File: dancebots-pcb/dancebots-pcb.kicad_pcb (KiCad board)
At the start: 2 copper layers, 50 x 50 mm, 33 parts, among them J1 BATTERY, J2 MOT2-L, J3 MOT1-R, J4 MP3 Player, U1 L4941, U2 L293, U3 ATTINY261A-P, U4 LM386, U5 LM358

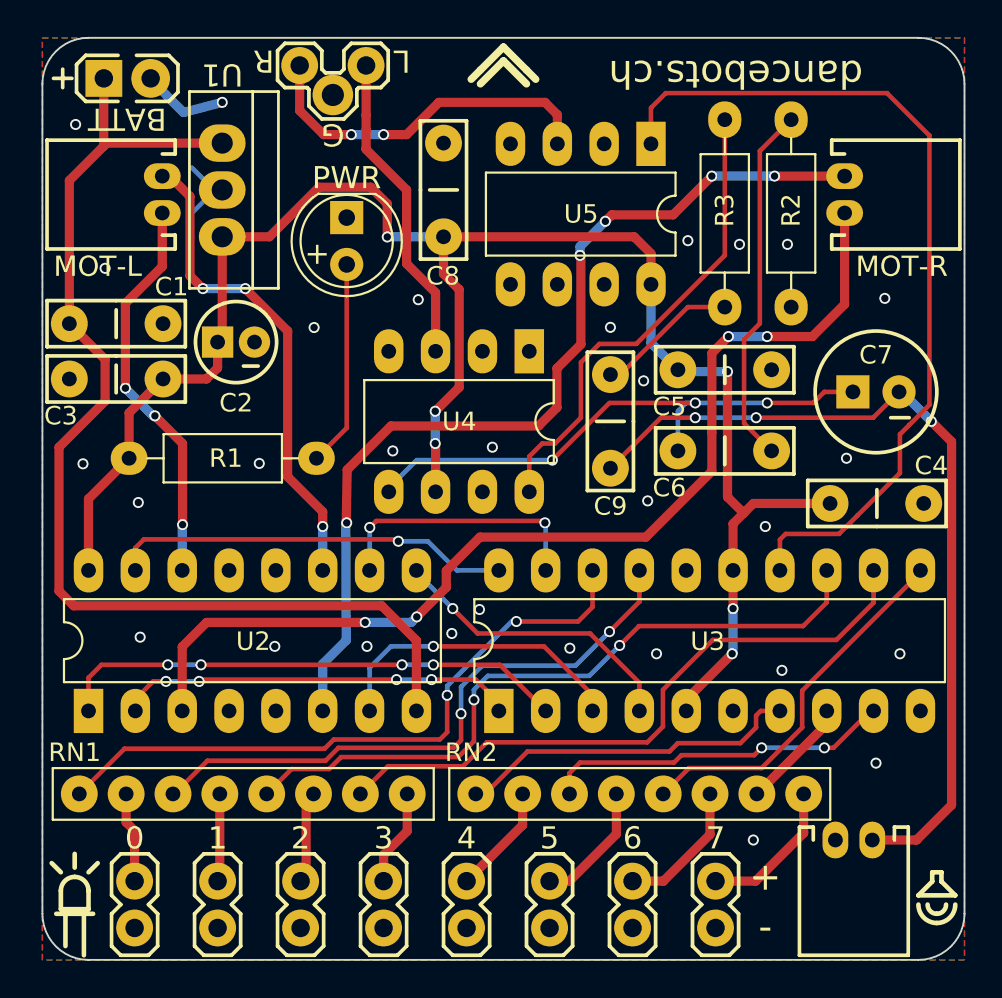
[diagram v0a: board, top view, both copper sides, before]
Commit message: migrated to Kicad 6.0
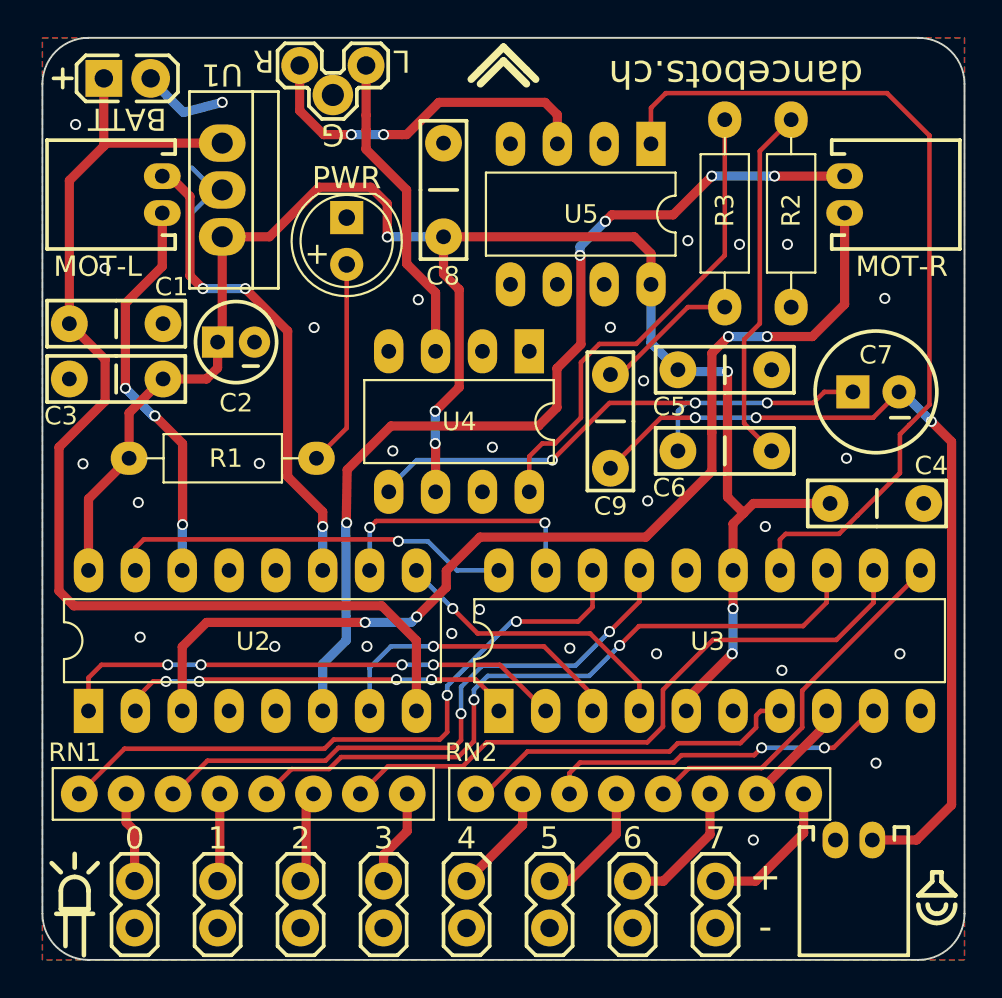
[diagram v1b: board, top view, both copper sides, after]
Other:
- net class Default removed
